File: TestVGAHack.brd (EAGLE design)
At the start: 70.1 x 24 mm, 0 parts

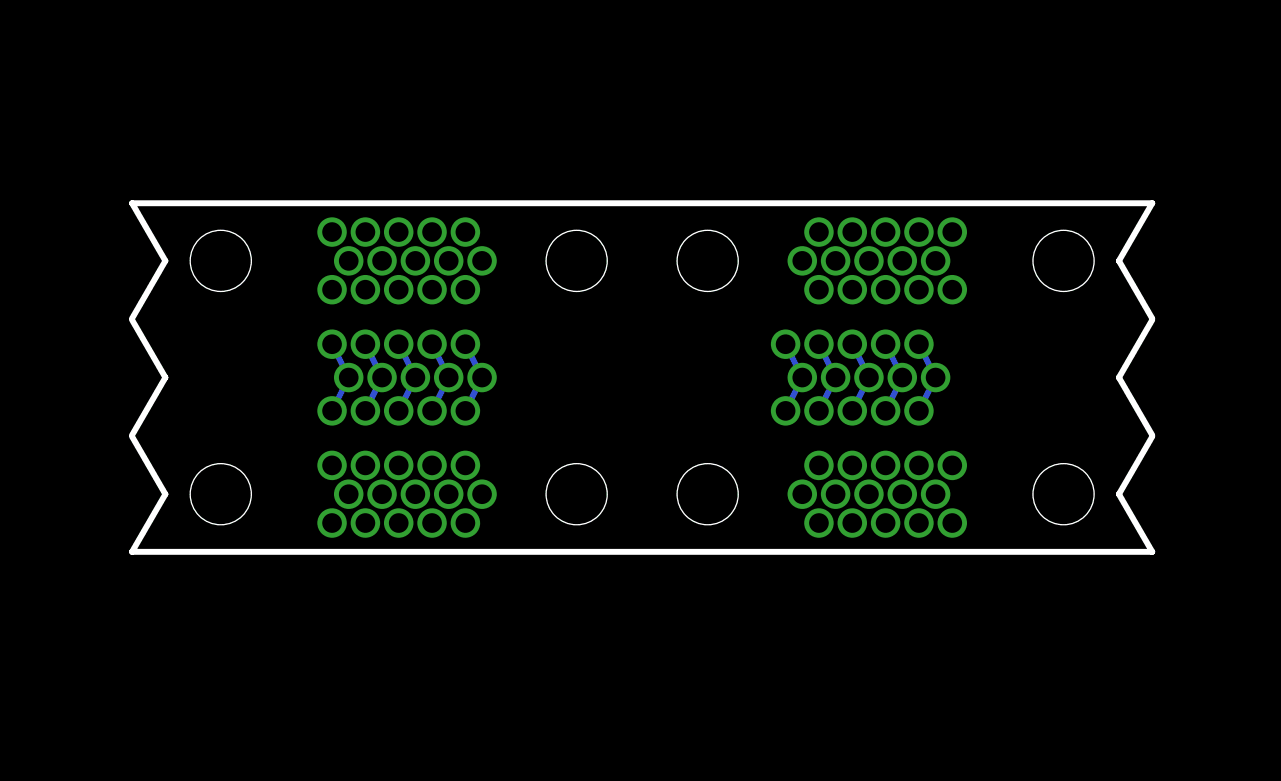
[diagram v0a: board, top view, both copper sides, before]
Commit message: Updated VGA hack board
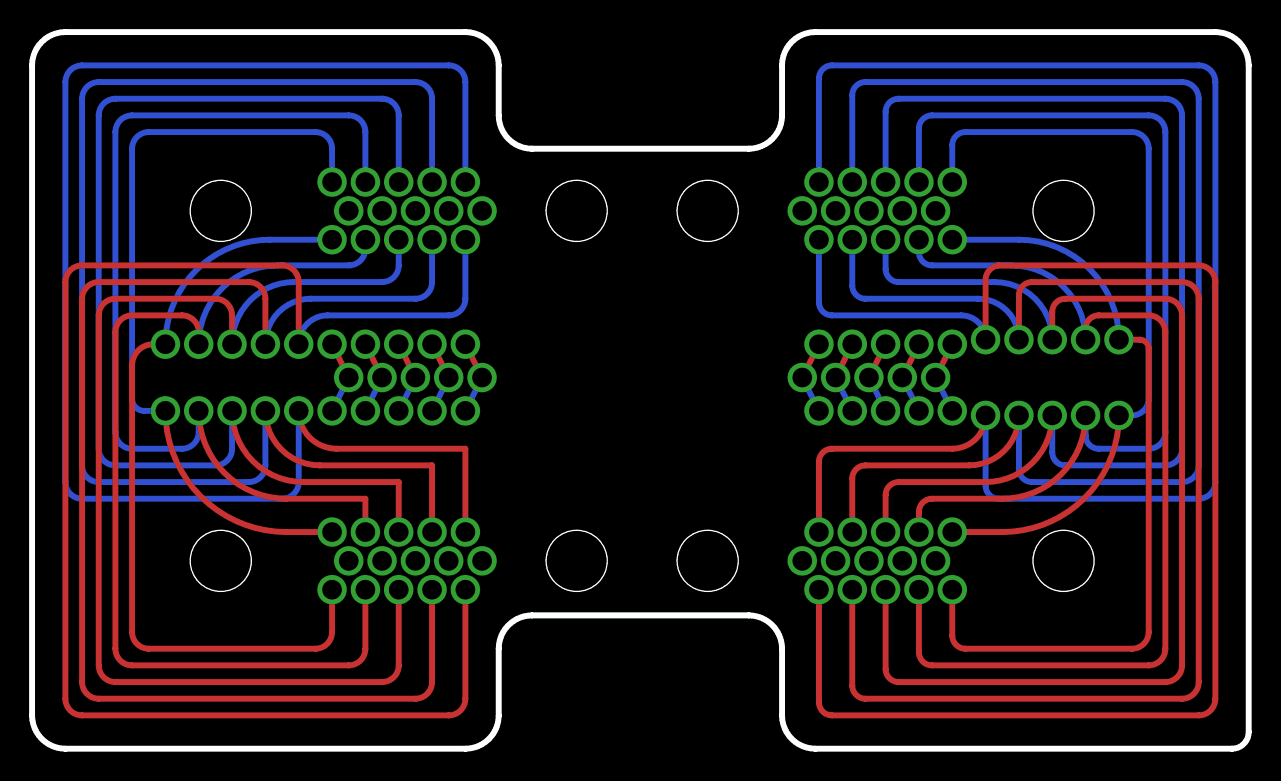
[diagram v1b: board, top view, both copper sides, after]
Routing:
- net C1: track 0.00 -> 102.9 mm, vias 2 -> 3
- net C11: track 0.00 -> 102.6 mm, vias 2 -> 3
- net C2_11: track 0.00 -> 102.0 mm, vias 2 -> 3
- net C2_1: track 0.00 -> 101.7 mm, vias 2 -> 3
- net C2: track 0.00 -> 90.8 mm, vias 2 -> 3
- net C12: track 0.00 -> 90.5 mm, vias 2 -> 3
- net C2_12: track 0.00 -> 90.0 mm, vias 2 -> 3
- net C2_2: track 0.00 -> 89.6 mm, vias 2 -> 3
- net C3: track 0.00 -> 78.7 mm, vias 2 -> 3
- net C13: track 0.00 -> 78.4 mm, vias 2 -> 3
- net C2_13: track 0.00 -> 77.9 mm, vias 2 -> 3
- net C2_3: track 0.00 -> 77.5 mm, vias 2 -> 3
- net C4: track 0.00 -> 66.5 mm, vias 2 -> 3
- net C14: track 0.00 -> 66.2 mm, vias 2 -> 3
- net C2_14: track 0.00 -> 65.7 mm, vias 2 -> 3
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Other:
- board size 70.1 x 24 mm -> 83.6 x 49.2 mm
